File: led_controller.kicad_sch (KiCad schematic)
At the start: 32 parts, among them IC1 ESP32-C3-MINI-1-N4X, IC2 L6983N33QTR, J1 Screw_Terminal_01x02, J2 Screw_Terminal_01x02, J3 Conn_01x04_Pin, J4 Screw_Terminal_01x02, J5 Conn_01x03_Pin, Q2 FQD13N10LTM

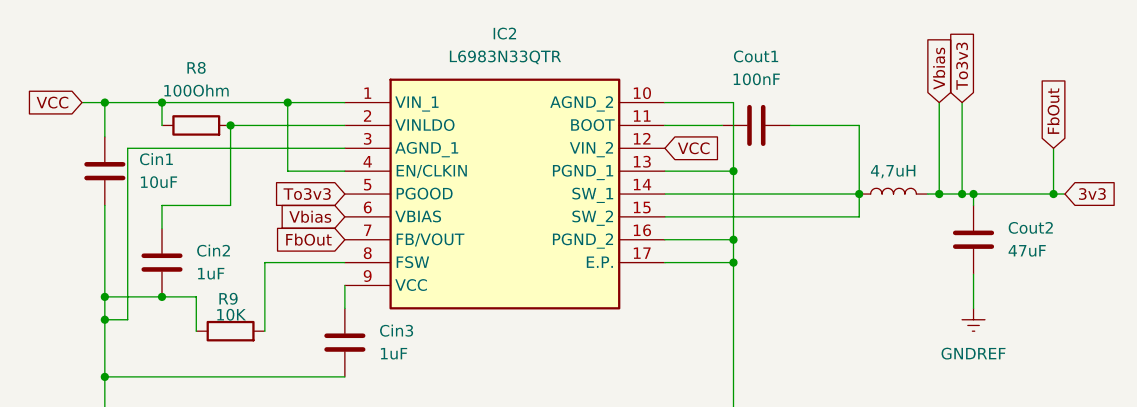
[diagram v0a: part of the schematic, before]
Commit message: Add files via upload
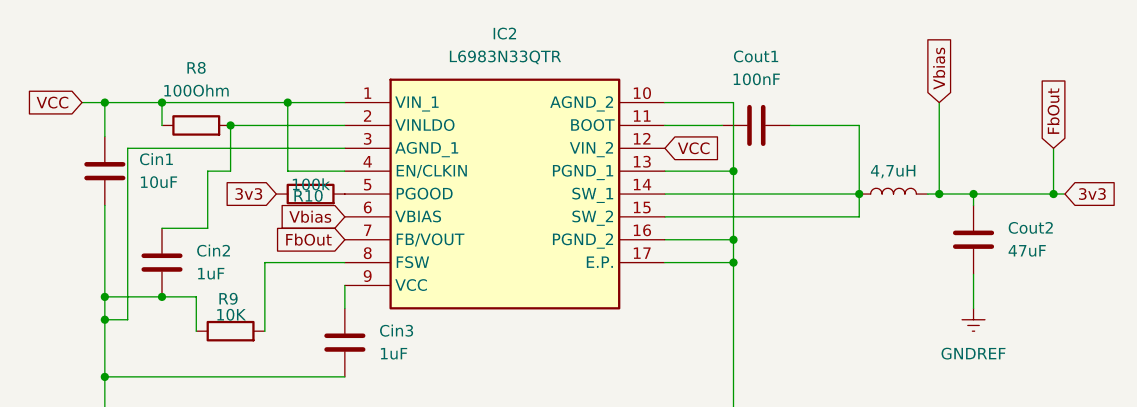
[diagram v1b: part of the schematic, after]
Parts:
- added R10: 100k, Resistor_SMD:R_0805_2012Metric_Pad1.20x1.40mm_HandSolder, symbol Device:R
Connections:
- net 3v3: now also R10.1; no longer IC2.5 (PGOOD)
- new net: IC2.5 (PGOOD), R10.2
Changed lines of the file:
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@@
 	)
 	(junction
-		(at 128.27 39.37)
-		(diameter 0)
-		(color 0 0 0 0)
-	)
-	(junction
 		(at 116.84 39.37)
 		(diameter 0)
@@
 	(wire
 		(pts
-			(xy 39.37 40.64) (xy 46.99 40.64)
+			(xy 39.37 43.18) (xy 44.45 43.18)
 		)
 		(stroke
@@
 	(wire
 		(pts
-			(xy 125.73 39.37) (xy 128.27 39.37)
+			(xy 125.73 39.37) (xy 129.54 39.37)
 		)
 		(stroke
@@
 	(wire
 		(pts
-			(xy 148.59 138.43) (xy 148.59 140.97)
+			(xy 46.99 36.83) (xy 46.99 31.75)
 		)
 		(stroke
@@
 	(wire
 		(pts
-			(xy 115.57 120.65) (xy 81.28 120.65)
+			(xy 148.59 138.43) (xy 148.59 140.97)
 		)
 		(stroke
@@
 	(wire
 		(pts
-			(xy 148.59 110.49) (xy 148.59 113.03)
+			(xy 115.57 120.65) (xy 81.28 120.65)
 		)
 		(stroke
@@
 	(wire
 		(pts
-			(xy 138.43 34.29) (xy 138.43 39.37)
+			(xy 148.59 110.49) (xy 148.59 113.03)
 		)
 		(stroke
@@
 	(wire
 		(pts
-			(xy 43.18 54.61) (xy 43.18 50.8)
+			(xy 138.43 34.29) (xy 138.43 39.37)
 		)
 		(stroke
@@
 	(wire
 		(pts
-			(xy 36.83 137.16) (xy 57.15 137.16)
+			(xy 43.18 54.61) (xy 43.18 50.8)
 		)
 		(stroke
@@
 	(wire
 		(pts
-			(xy 184.15 59.69) (xy 189.23 59.69)
+			(xy 36.83 137.16) (xy 57.15 137.16)
 		)
 		(stroke
@@
 	(wire
 		(pts
-			(xy 128.27 39.37) (xy 129.54 39.37)
+			(xy 184.15 59.69) (xy 189.23 59.69)
 		)
 		(stroke
@@
 	(wire
 		(pts
-			(xy 209.55 128.27) (xy 209.55 137.16)
+			(xy 44.45 36.83) (xy 46.99 36.83)
 		)
 		(stroke
@@
 	(wire
 		(pts
-			(xy 104.14 100.33) (xy 115.57 100.33)
+			(xy 209.55 128.27) (xy 209.55 137.16)
 		)
 		(stroke
@@
 	(wire
 		(pts
-			(xy 109.22 31.75) (xy 116.84 31.75)
+			(xy 104.14 100.33) (xy 115.57 100.33)
 		)
 		(stroke
@@
 	(wire
 		(pts
-			(xy 128.27 29.21) (xy 128.27 39.37)
+			(xy 109.22 31.75) (xy 116.84 31.75)
 		)
 		(stroke
@@
 	(wire
 		(pts
-			(xy 39.37 43.18) (xy 39.37 40.64)
-		)
-		(stroke
-			(width 0)
-			(type default)
-		)
-	)
-	(wire
-		(pts
 			(xy 205.74 118.11) (xy 205.74 119.38)
 		)
@@
 	(wire
 		(pts
-			(xy 46.99 31.75) (xy 46.99 40.64)
+			(xy 44.45 36.83) (xy 44.45 43.18)
 		)
 		(stroke
@@
 		)
 	)
-	(global_label "VCC"
+	(global_label "3v3"
 		(shape input)
-		(at 189.23 57.15 90)
+		(at 52.07 39.37 180)
 		(fields_autoplaced yes)
 		(effects
@@
 				(size 1.27 1.27)
 			)
-			(justify left)
+			(justify right)
 		)
 		(property "Intersheetrefs" "${INTERSHEET_REFS}"
-			(at 189.23 50.5362 90)
+			(at 45.6982 39.37 0)
 			(effects
 				(font
 					(size 1.27 1.27)
 				)
-				(justify left)
+				(justify right)
 				(hide yes)
 			)
 		)
 	)
-	(global_label "3v3"
+	(global_label "VCC"
 		(shape input)
-		(at 27.94 143.51 180)
+		(at 189.23 57.15 90)
 		(fields_autoplaced yes)
 		(effects
@@
 				(size 1.27 1.27)
 			)
-			(justify right)
+			(justify left)
 		)
 		(property "Intersheetrefs" "${INTERSHEET_REFS}"
-			(at 21.5682 143.51 0)
+			(at 189.23 50.5362 90)
 			(effects
 				(font
 					(size 1.27 1.27)
 				)
-				(justify right)
+				(justify left)
 				(hide yes)
 			)
 		)
 	)
-	(global_label "To3v3"
+	(global_label "3v3"
 		(shape input)
-		(at 128.27 29.21 90)
+		(at 27.94 143.51 180)
 		(fields_autoplaced yes)
 		(effects
@@
 				(size 1.27 1.27)
 			)
-			(justify left)
+			(justify right)
 		)
 		(property "Intersheetrefs" "${INTERSHEET_REFS}"
-			(at 128.27 20.7216 90)
+			(at 21.5682 143.51 0)
 			(effects
 				(font
 					(size 1.27 1.27)
 				)
-				(justify left)
+				(justify right)
 				(hide yes)
 			)
@@
 		)
 	)
-	(global_label "To3v3"
-		(shape input)
-		(at 59.69 39.37 180)
-		(fields_autoplaced yes)
-		(effects
-			(font
-				(size 1.27 1.27)
-			)
-			(justify right)
-		)
-		(property "Intersheetrefs" "${INTERSHEET_REFS}"
-			(at 51.2016 39.37 0)
-			(effects
-				(font
-					(size 1.27 1.27)
-				)
-				(justify right)
-				(hide yes)
-			)
-		)
-	)
 	(global_label "IO5"
 		(shape input)
@@
 					(unit 1)
 				)
+			)
+		)
+	)
+	(symbol
+		(lib_id "Device:R")
+		(at 55.88 39.37 90)
+		(unit 1)
+		(exclude_from_sim no)
+		(in_bom yes)
+		(on_board yes)
+		(dnp no)
+		(property "Reference" "R10"
+			(at 55.626 39.624 90)
+			(effects
+				(font
+					(size 1.27 1.27)
+				)
+			)
+		)
+		(property "Value" "100k"
+			(at 55.88 38.354 90)
+			(effects
+				(font
+					(size 1.27 1.27)
+				)
+			)
+		)
+		(property "Footprint" "Resistor_SMD:R_0805_2012Metric_Pad1.20x1.40mm_HandSolder"
+			(at 55.88 41.148 90)
+			(effects
+				(font
+					(size 1.27 1.27)
+				)
+				(hide yes)
+			)
+		)
+		(property "Datasheet" "~"
+			(at 55.88 39.37 0)
+			(effects
+				(font
+					(size 1.27 1.27)
+				)
+				(hide yes)
+			)
+		)
+		(property "Description" "Resistor"
+			(at 55.88 39.37 0)
+			(effects
+				(font
+					(size 1.27 1.27)
+				)
+				(hide yes)
+			)
+		)
+		(pin "1"
+		)
+		(pin "2"
+		)
+		(instances
+			(project "led_controller"
+				(path "/f7384fac-022b-47e0-8e4e-5c549011b8cf"
+					(reference "R10")
+					(unit 1)
+				)
